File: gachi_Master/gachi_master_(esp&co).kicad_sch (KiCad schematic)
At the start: 1 part

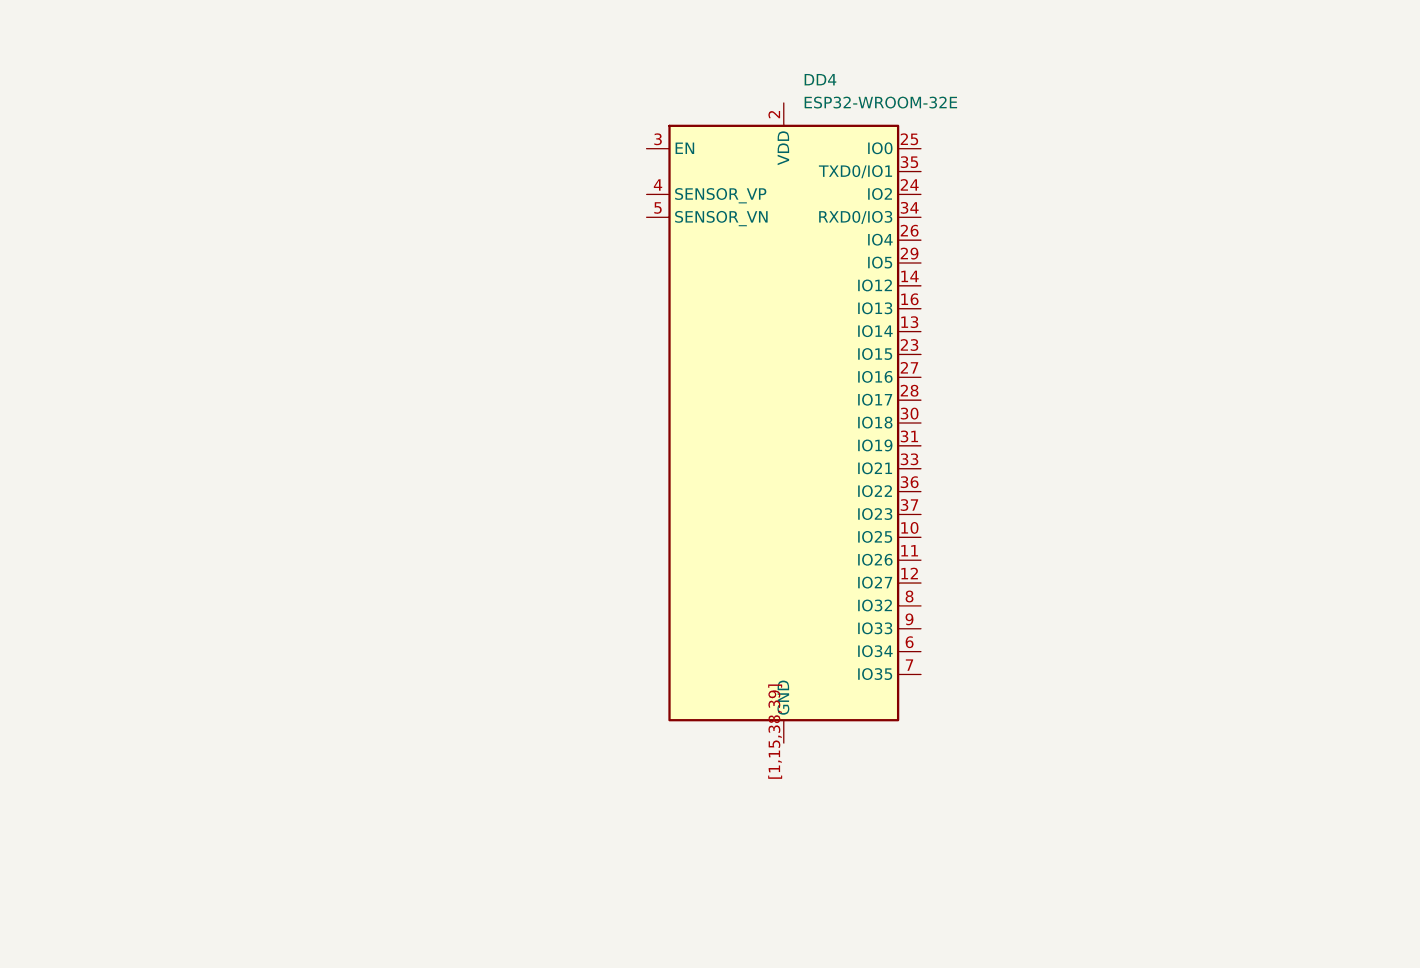
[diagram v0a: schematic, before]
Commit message: update_10.10.2026_2
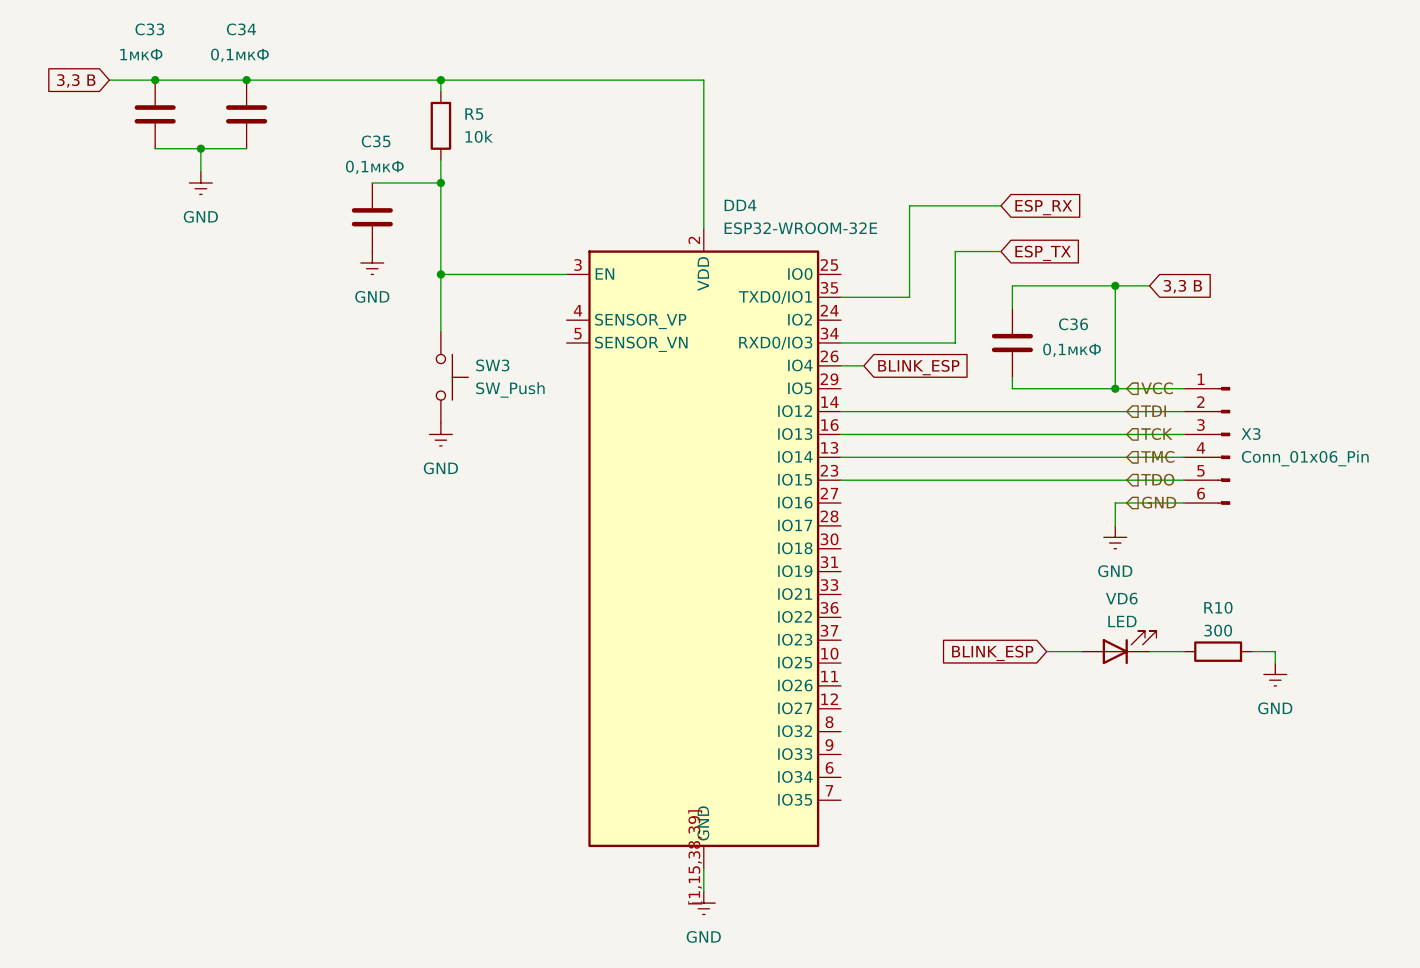
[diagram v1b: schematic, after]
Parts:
- added C33: 1мкФ, Capacitor_SMD:C_0603_1608Metric, symbol Device:C
- added C34, C35, C36: 0,1мкФ, Capacitor_SMD:C_0603_1608Metric, symbol Device:C
- added R10: 300, Resistor_SMD:R_0603_1608Metric, symbol Device:R
- added R5: 10k, Resistor_SMD:R_0603_1608Metric, symbol Device:R
- added SW3: SW_Push, symbol Switch:SW_Push
- added VD6: LED, LED_SMD:LED_0603_1608Metric, symbol Device:LED
- added X3: Conn_01x06_Pin, Connector:Tag-Connect_TC2030-IDC-FP_2x03_P1.27mm_Vertical, symbol Connector:Conn_01x06_Pin
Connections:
- net TMC: now reaches DD4.13 (IO14)
- net TMC: now also X3.4 (Pin_4)
- net TDI: now reaches DD4.14 (IO12)
- net TDI: now also X3.2 (Pin_2)
- net TCK: now reaches DD4.16 (IO13)
- net TCK: now also X3.3 (Pin_3)
- net 3,3 В: now reaches DD4.2 (VDD)
- net 3,3 В: now also C33.1, C34.1, C36.1, C36.2, R5.2, X3.1 (Pin_1)
- net TDO: now reaches DD4.23 (IO15)
- net TDO: now also X3.5 (Pin_5)
- net BLINK_ESP: now reaches DD4.26 (IO4)
- net BLINK_ESP: now also VD6.2 (A)
- net at DD4.3 (EN): now also C35.1, R5.1, SW3.1
- net ESP_TX: now reaches DD4.34 (RXD0/IO3)
- net ESP_RX: now reaches DD4.35 (TXD0/IO1)
- net GND: now reaches DD4.[1,15,38,39] (GND)
- net GND: now also C33.2, C34.2, C35.2, R10.2, SW3.2, X3.6 (Pin_6)
- new net: R10.1, VD6.1 (K)
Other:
- moved on the sheet: DD4
